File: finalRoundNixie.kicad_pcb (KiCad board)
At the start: 2 copper layers, 37 x 56.3 mm, 60 parts, among them J1 Conn_01x06_Male, J2 HV_IN, J3 Conn_01x06_Female, J4 HV_OUT, Q1 MMBTA42LT1, Q10 MMBTA42LT1, Q11 AO3400, Q12 AO3400, Q13 AO3400, Q14 MMBTA42LT1, Q15 MMBTA42LT1, Q2 MMBTA42LT1, Q3 MMBTA42LT1, Q4 MMBTA42LT1, Q5 MMBTA42LT1, Q6 MMBTA42LT1, Q7 MMBTA42LT1, Q8 MMBTA42LT1, Q9 MMBTA42LT1, U1 74HC595D, U2 nixie-tube, U3 74HC595D, U4 ams1117-5.0

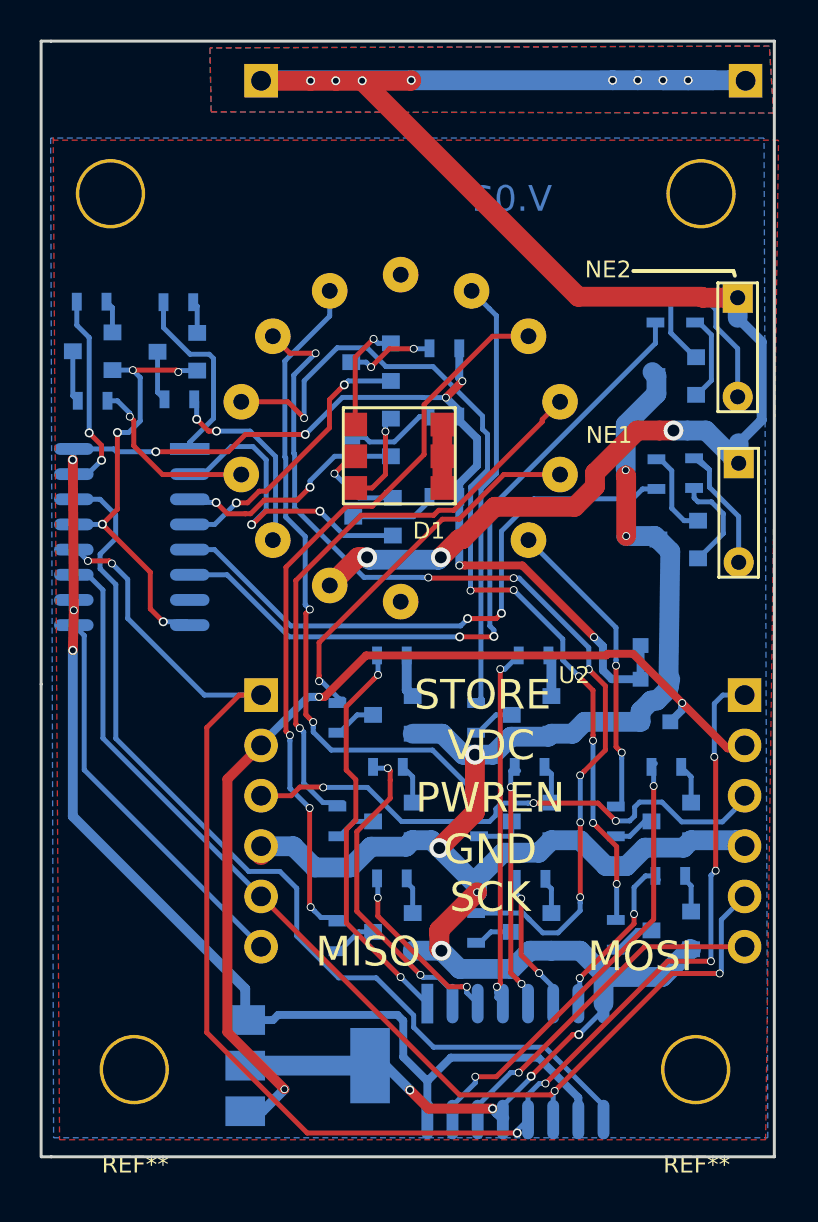
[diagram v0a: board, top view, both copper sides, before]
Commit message: finalized tracks and added symbols
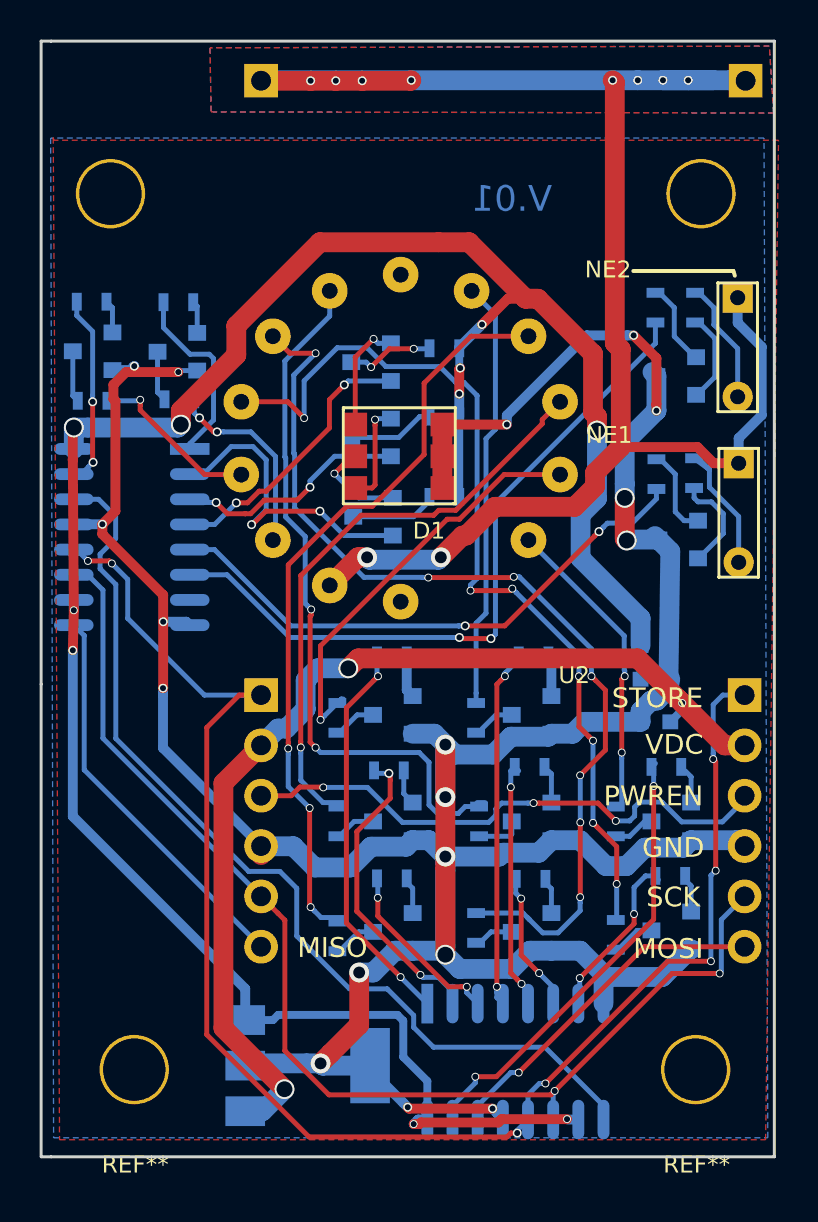
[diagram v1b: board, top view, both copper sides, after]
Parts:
- moved R18 0.18 mm to (169.1, 77.1)
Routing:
- net GND: track 139.9 -> 177.7 mm, vias 15 -> 18
- net +5V: track 103.0 -> 122.0 mm, vias 9 -> 10
- net Net-(J2-Pad1): track 91.9 -> 86.4 mm, vias 11 -> 10
- net /SCK: track 56.3 -> 60.1 mm
- net +VDC: track 51.6 -> 54.8 mm
- net /DotU: track 30.4 -> 28.3 mm
- net Net-(R5-Pad1): track 34.1 -> 36.1 mm
- net Net-(R9-Pad1): track 19.2 -> 21.0 mm
- net Net-(R2-Pad1): track 9.34 -> 8.64 mm
- net /s8: track 10.8 -> 10.2 mm
- net Net-(R7-Pad1): track 38.1 -> 38.6 mm
